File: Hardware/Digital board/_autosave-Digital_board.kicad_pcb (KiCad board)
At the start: 4 copper layers, 100 x 100 mm, 122 parts, among them P1 CONN_01X04, P2 1MHz osc, P3 DIL18, P4 CONN_02X13, P5 CONN_02X13, P6 CONN_02X13, P7 CONN_02X13, P8 CONN_01X02, U1 74LS32, U10 SST39SF020, U11 74LS541, U12 Dip-mem_2Mx8b, U13 4040, U14 74LS541, U15 74LS02, U16 74LS373, U17 74LS32, U18 DAC08, U19 MCP1541-I/TO, U2 74LS21, U20 74LS373, U21 74HC138, U22 TL074, U23 74LS541, U24 4040, U25 74LS163, U26 SST39SF020, U27 74LS21, U28 74LS21, U29 74LS373, U3 4040, U31 4040, U32 DAC08, U33 TL074, U34 LM386, U4 4040, U5 4040, U6 4040, U7 74LS08, U8 74LS373, U9 SST39SF020

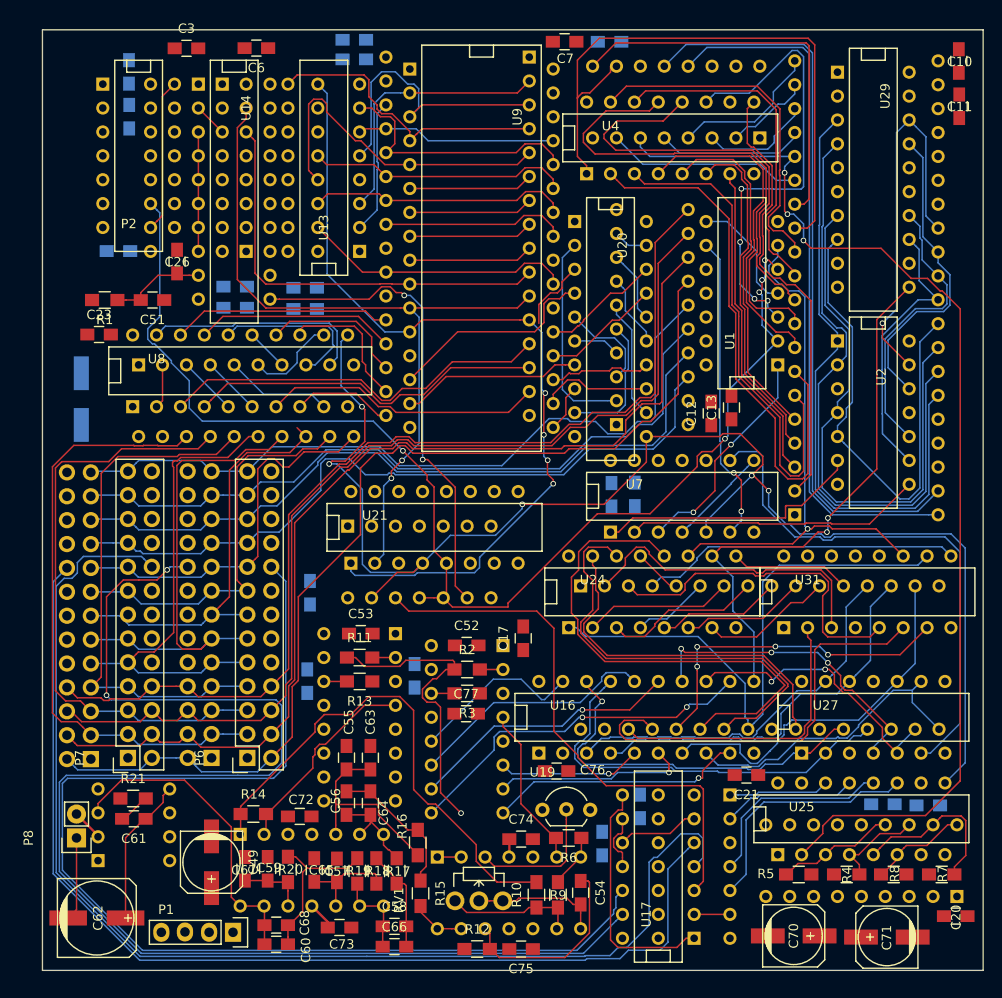
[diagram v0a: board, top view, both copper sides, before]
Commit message: Pcb design
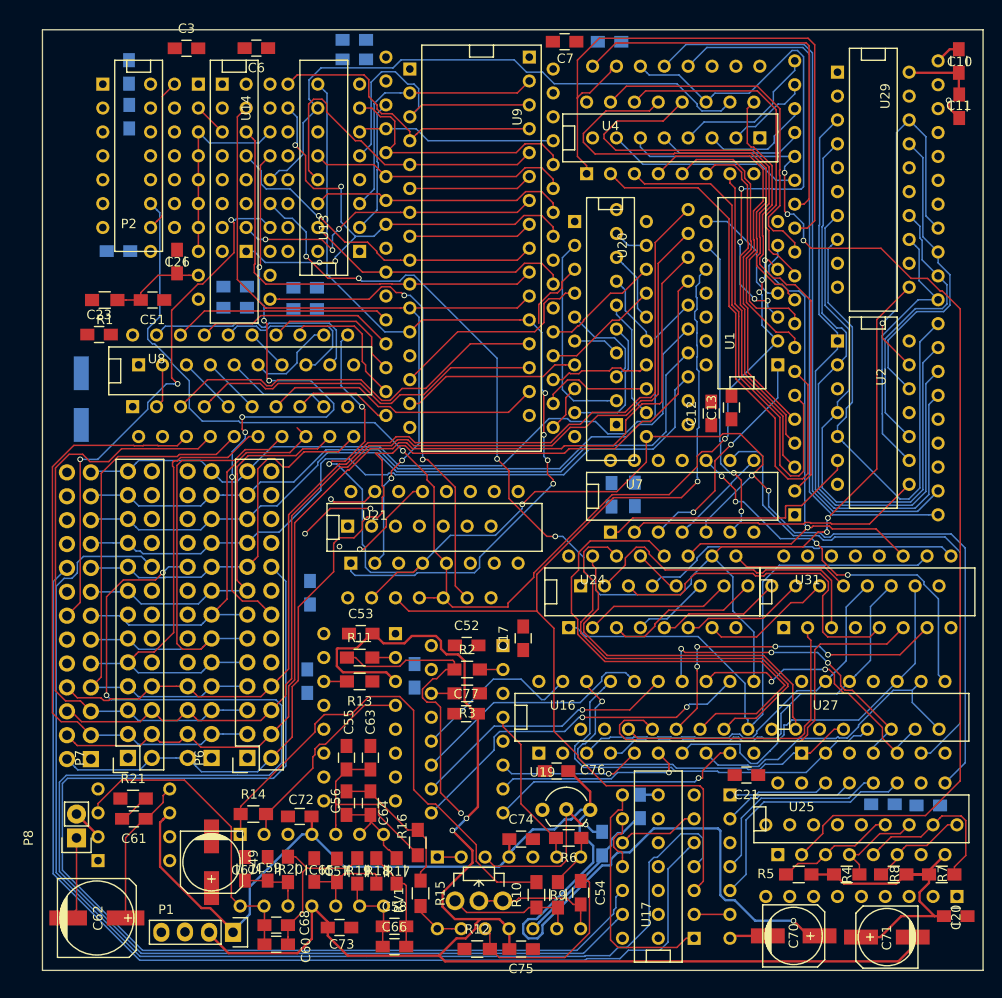
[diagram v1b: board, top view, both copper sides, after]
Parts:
- turned C11 to 270 degrees
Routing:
- net -12VA: track 2.99 -> 157.0 mm, vias 0 -> 2
- net +12VA: track 1.92 -> 138.1 mm, vias 0 -> 1
- net /Clk_main3: track 58.1 -> 135.8 mm, vias 2 -> 6
- net /Clk_main7: track 0.00 -> 67.8 mm, vias 0 -> 6
- net GND: track 3.36 -> 67.7 mm, vias 0 -> 1
- net /Clk_main2: track 0.00 -> 62.0 mm
- net /Clk_main4: track 0.00 -> 56.8 mm, vias 0 -> 3
- net /Rst_Gam: track 58.9 -> 107.4 mm, vias 0 -> 1
- net /Clk_main5: track 0.00 -> 47.4 mm
- net /Clk_main6: track 0.00 -> 44.5 mm
- net /RST_GM0: track 0.00 -> 41.6 mm, vias 0 -> 1
- net Net-(U27-Pad8): track 0.00 -> 41.5 mm, vias 0 -> 4
- net /Clk_gme_data: track 19.7 -> 55.8 mm, vias 0 -> 4
- net /RST_GM1: track 0.00 -> 35.9 mm, vias 0 -> 2
- net /RST_GM2: track 0.00 -> 31.4 mm, vias 0 -> 2
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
